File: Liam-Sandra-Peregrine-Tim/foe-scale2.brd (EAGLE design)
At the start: 96.2 x 67.3 mm, 53 parts, among them U1 LM311, U2 SAMD21E

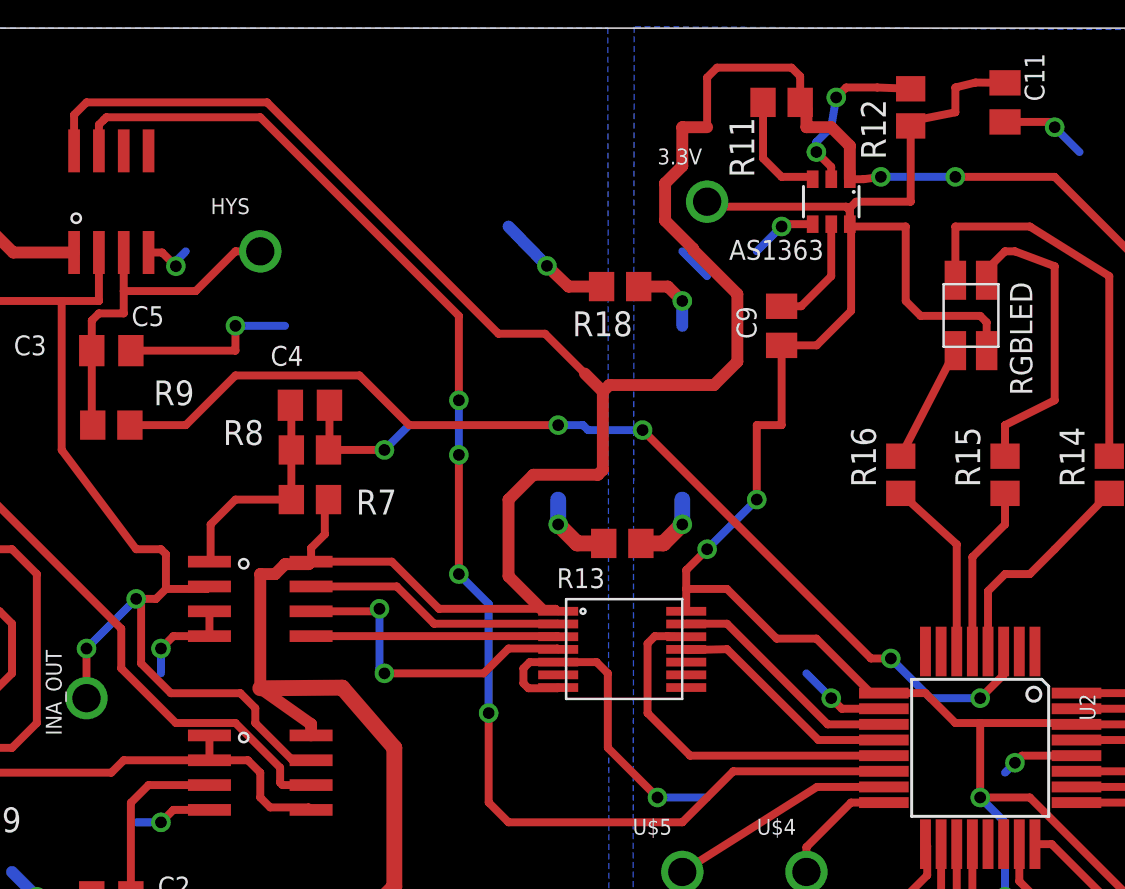
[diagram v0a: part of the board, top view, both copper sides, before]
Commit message: pushing
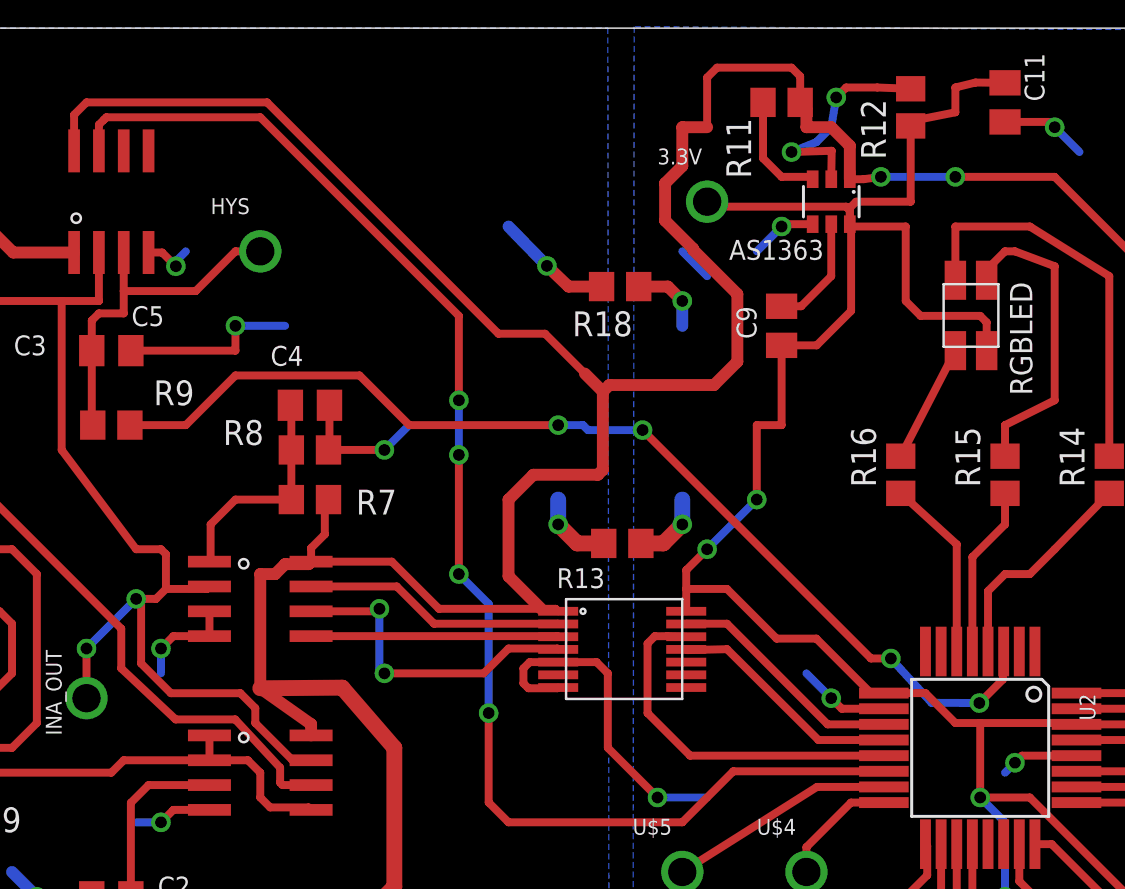
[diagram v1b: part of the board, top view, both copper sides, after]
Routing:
- net N$70: track 8.86 -> 11.5 mm
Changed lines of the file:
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@@
 </class>
 </classes>
-<designrules name="default">
+<designrules name="default *">
 <description language="de">&lt;b&gt;EAGLE Design Rules&lt;/b&gt;
 &lt;p&gt;
@@
 <param name="mtCopper" value="0.035mm 0.035mm 0.035mm 0.035mm 0.035mm 0.035mm 0.035mm 0.035mm 0.035mm 0.035mm 0.035mm 0.035mm 0.035mm 0.035mm 0.035mm 0.035mm"/>
 <param name="mtIsolate" value="1.5mm 0.15mm 0.2mm 0.15mm 0.2mm 0.15mm 0.2mm 0.15mm 0.2mm 0.15mm 0.2mm 0.15mm 0.2mm 0.15mm 0.2mm"/>
-<param name="mdWireWire" value="8mil"/>
-<param name="mdWirePad" value="8mil"/>
-<param name="mdWireVia" value="8mil"/>
-<param name="mdPadPad" value="8mil"/>
-<param name="mdPadVia" value="8mil"/>
-<param name="mdViaVia" value="8mil"/>
-<param name="mdSmdPad" value="8mil"/>
-<param name="mdSmdVia" value="8mil"/>
-<param name="mdSmdSmd" value="8mil"/>
+<param name="mdWireWire" value="6mil"/>
+<param name="mdWirePad" value="6mil"/>
+<param name="mdWireVia" value="6mil"/>
+<param name="mdPadPad" value="6mil"/>
+<param name="mdPadVia" value="6mil"/>
+<param name="mdViaVia" value="6mil"/>
+<param name="mdSmdPad" value="6mil"/>
+<param name="mdSmdVia" value="6mil"/>
+<param name="mdSmdSmd" value="6mil"/>
 <param name="mdViaViaSameLayer" value="8mil"/>
 <param name="mnLayersViaInSmd" value="2"/>
 <param name="mdCopperDimension" value="40mil"/>
-<param name="mdDrill" value="8mil"/>
+<param name="mdDrill" value="6mil"/>
 <param name="mdSmdStop" value="0mil"/>
 <param name="msWidth" value="10mil"/>
@@
 </element>
 <element name="R11" library="resistor" package="R0805" value="10k" x="63.5" y="76.2" smashed="yes" rot="R180">
-<attribute name="NAME" x="60.833" y="75.438" size="1.27" layer="25" rot="R270"/>
+<attribute name="NAME" x="60.671525" y="75.39493125" size="1.27" layer="25" rot="R270"/>
 <attribute name="VALUE" x="61.849" y="78.232" size="1.27" layer="27"/>
 </element>
@@
 <wire x1="37.973" y1="41.275" x2="37.846" y2="41.402" width="0.4064" layer="1"/>
 <wire x1="37.846" y1="41.402" x2="37.846" y2="42.164" width="0.4064" layer="1"/>
-<wire x1="37.846" y1="42.164" x2="35.56" y2="44.45" width="0.4064" layer="1"/>
-<wire x1="35.56" y1="44.45" x2="32.512" y2="44.45" width="0.4064" layer="1"/>
-<wire x1="32.512" y1="44.45" x2="29.718" y2="47.244" width="0.4064" layer="1"/>
+<wire x1="37.846" y1="42.164" x2="35.549234375" y2="44.633034375" width="0.4064" layer="1"/>
+<wire x1="35.549234375" y1="44.633034375" x2="32.501234375" y2="44.633034375" width="0.4064" layer="1"/>
+<wire x1="32.501234375" y1="44.633034375" x2="29.718" y2="47.244" width="0.4064" layer="1"/>
 <wire x1="29.718" y1="47.244" x2="29.718" y2="49.276" width="0.4064" layer="1"/>
 <wire x1="29.718" y1="49.276" x2="22.606" y2="56.388" width="0.4064" layer="1"/>
@@
 <contactref element="U2" pad="3"/>
 <wire x1="30.16" y1="59.69" x2="30.48" y2="59.69" width="0.4064" layer="1"/>
-<wire x1="74.86" y1="48.1076" x2="74.86" y2="46.92" width="0.4064" layer="1"/>
-<wire x1="74.86" y1="46.92" x2="73.66" y2="45.72" width="0.4064" layer="1"/>
-<via x="73.66" y="45.72" extent="1-16" drill="0.6"/>
-<wire x1="73.66" y1="45.72" x2="71.12" y2="45.72" width="0.4064" layer="16"/>
-<wire x1="71.12" y1="45.72" x2="69.088" y2="47.752" width="0.4064" layer="16"/>
+<wire x1="74.86" y1="48.1076" x2="74.816940625" y2="46.672365625" width="0.4064" layer="1"/>
+<wire x1="74.816940625" y1="46.672365625" x2="73.616940625" y2="45.472365625" width="0.4064" layer="1"/>
+<via x="73.616940625" y="45.472365625" extent="1-16" drill="0.6"/>
+<wire x1="73.616940625" y1="45.472365625" x2="71.173825" y2="45.48313125" width="0.4064" layer="16"/>
+<wire x1="71.173825" y1="45.48313125" x2="69.088" y2="47.752" width="0.4064" layer="16"/>
 <via x="69.088" y="47.752" extent="1-16" drill="0.6"/>
 <wire x1="69.088" y1="47.752" x2="68.072" y2="47.752" width="0.4064" layer="1"/>
@@
 <contactref element="R12" pad="2"/>
 <contactref element="AS1363" pad="2"/>
-<wire x1="66.04" y1="72.27" x2="66.04" y2="72.898" width="0.4064" layer="1"/>
-<wire x1="66.04" y1="72.898" x2="65.278" y2="73.66" width="0.4064" layer="1"/>
-<via x="65.278" y="73.66" extent="1-16" drill="0.6"/>
-<wire x1="65.278" y1="73.66" x2="65.278" y2="74.168" width="0.4064" layer="16"/>
+<wire x1="66.04" y1="72.27" x2="66.06233125" y2="73.724378125" width="0.4064" layer="1"/>
+<wire x1="66.06233125" y1="73.724378125" x2="64.008" y2="73.66" width="0.4064" layer="1"/>
+<via x="64.008" y="73.66" extent="1-16" drill="0.6"/>
+<wire x1="64.008" y1="73.66" x2="65.278" y2="74.168" width="0.4064" layer="16"/>
 <wire x1="65.278" y1="74.168" x2="66.04" y2="74.93" width="0.4064" layer="16"/>
 <wire x1="66.04" y1="74.93" x2="66.294" y2="76.454" width="0.4064" layer="16"/>
